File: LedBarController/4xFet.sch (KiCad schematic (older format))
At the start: 4 parts, among them Q301 Si2302DS, Q302 Si2302DS, Q303 Si2302DS, Q304 Si2302DS

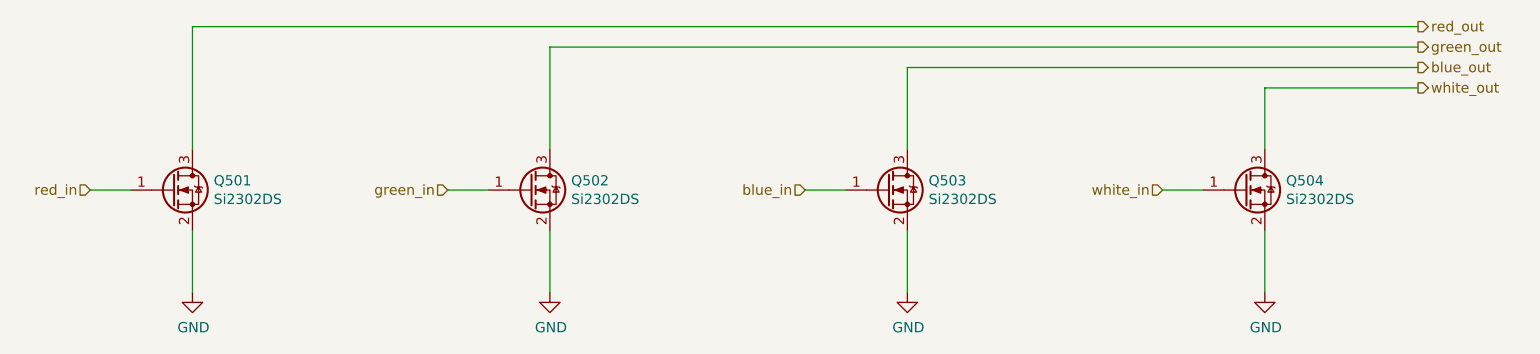
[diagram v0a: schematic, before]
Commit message: Just before reverse order of strips
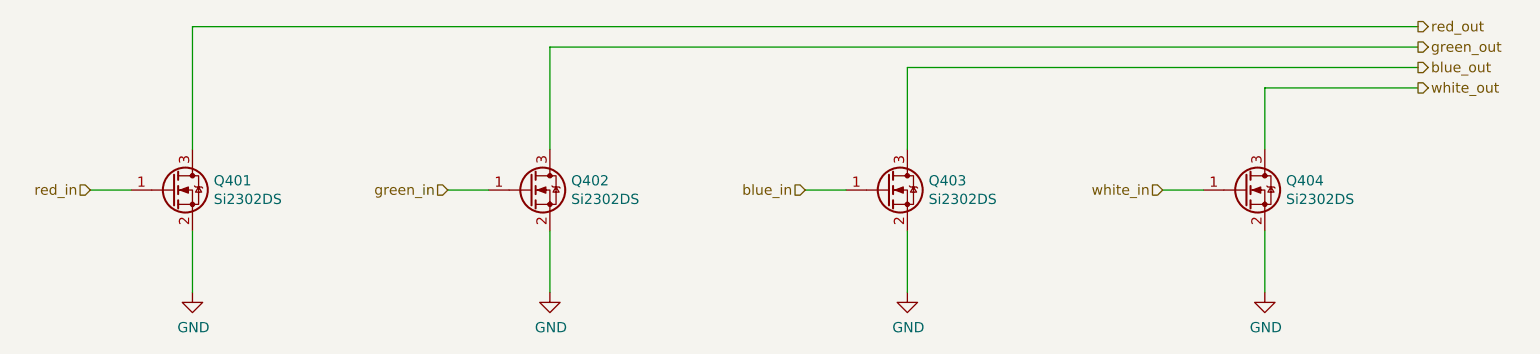
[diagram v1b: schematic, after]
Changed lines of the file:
@@
 $Descr A4 11693 8268
 encoding utf-8
-Sheet 5 13
+Sheet 4 13
 Title ""
 Date ""
@@
 AR Path="/5F8F2E1B/5F902D83/5F88FE87" Ref="#PWR0504"  Part="1"
 AR Path="/5F8F2E1B/5F902E61/5F88FE87" Ref="#PWR0604"  Part="1"
-F 0 "#PWR0604" H 7750 4050 50  0001 C CNN
+F 0 "#PWR0404" H 7750 4050 50  0001 C CNN
 F 1 "GND" H 7755 4127 50  0000 C CNN
 F 2 "" H 7750 4300 50  0001 C CNN
@@
 AR Path="/5F8F2E1B/5F902D83/5F88FE81" Ref="Q504"  Part="1"
 AR Path="/5F8F2E1B/5F902E61/5F88FE81" Ref="Q604"  Part="1"
-F 0 "Q504" H 7854 3846 50  0000 L CNN
+F 0 "Q404" H 7854 3846 50  0000 L CNN
 F 1 "Si2302DS" H 7854 3755 50  0000 L CNN
 F 2 "Package_TO_SOT_SMD:SOT-23_Handsoldering" H 7850 3900 50  0001 C CNN
@@
 AR Path="/5F8F2E1B/5F902D83/5F88FE79" Ref="#PWR0503"  Part="1"
 AR Path="/5F8F2E1B/5F902E61/5F88FE79" Ref="#PWR0603"  Part="1"
-F 0 "#PWR0603" H 6000 4050 50  0001 C CNN
+F 0 "#PWR0403" H 6000 4050 50  0001 C CNN
 F 1 "GND" H 6005 4127 50  0000 C CNN
 F 2 "" H 6000 4300 50  0001 C CNN
@@
 AR Path="/5F8F2E1B/5F902D83/5F88FE73" Ref="Q503"  Part="1"
 AR Path="/5F8F2E1B/5F902E61/5F88FE73" Ref="Q603"  Part="1"
-F 0 "Q503" H 6104 3846 50  0000 L CNN
+F 0 "Q403" H 6104 3846 50  0000 L CNN
 F 1 "Si2302DS" H 6104 3755 50  0000 L CNN
 F 2 "Package_TO_SOT_SMD:SOT-23_Handsoldering" H 6100 3900 50  0001 C CNN
@@
 AR Path="/5F8F2E1B/5F902D83/5F88FE6B" Ref="#PWR0502"  Part="1"
 AR Path="/5F8F2E1B/5F902E61/5F88FE6B" Ref="#PWR0602"  Part="1"
-F 0 "#PWR0602" H 4250 4050 50  0001 C CNN
+F 0 "#PWR0402" H 4250 4050 50  0001 C CNN
 F 1 "GND" H 4255 4127 50  0000 C CNN
 F 2 "" H 4250 4300 50  0001 C CNN
@@
 AR Path="/5F8F2E1B/5F902D83/5F88FE65" Ref="Q502"  Part="1"
 AR Path="/5F8F2E1B/5F902E61/5F88FE65" Ref="Q602"  Part="1"
-F 0 "Q502" H 4354 3846 50  0000 L CNN
+F 0 "Q402" H 4354 3846 50  0000 L CNN
 F 1 "Si2302DS" H 4354 3755 50  0000 L CNN
 F 2 "Package_TO_SOT_SMD:SOT-23_Handsoldering" H 4350 3900 50  0001 C CNN
@@
 AR Path="/5F8F2E1B/5F902D83/5F88FE5E" Ref="#PWR0501"  Part="1"
 AR Path="/5F8F2E1B/5F902E61/5F88FE5E" Ref="#PWR0601"  Part="1"
-F 0 "#PWR0601" H 2500 4050 50  0001 C CNN
+F 0 "#PWR0401" H 2500 4050 50  0001 C CNN
 F 1 "GND" H 2505 4127 50  0000 C CNN
 F 2 "" H 2500 4300 50  0001 C CNN
@@
 AR Path="/5F8F2E1B/5F902D83/5F88FE58" Ref="Q501"  Part="1"
 AR Path="/5F8F2E1B/5F902E61/5F88FE58" Ref="Q601"  Part="1"
-F 0 "Q501" H 2604 3846 50  0000 L CNN
+F 0 "Q401" H 2604 3846 50  0000 L CNN
 F 1 "Si2302DS" H 2604 3755 50  0000 L CNN
 F 2 "Package_TO_SOT_SMD:SOT-23_Handsoldering" H 2600 3900 50  0001 C CNN

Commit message: Before moving down the center connector
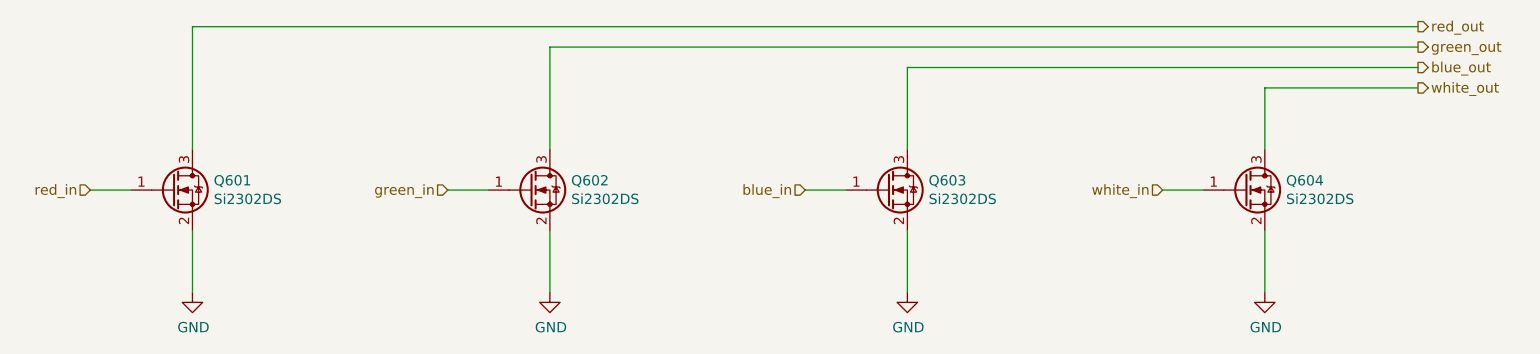
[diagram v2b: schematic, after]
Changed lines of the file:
@@
 $Descr A4 11693 8268
 encoding utf-8
-Sheet 4 13
+Sheet 6 13
 Title ""
 Date ""
@@
 AR Path="/5F8F2E1B/5F902D83/5F88FE87" Ref="#PWR0504"  Part="1"
 AR Path="/5F8F2E1B/5F902E61/5F88FE87" Ref="#PWR0604"  Part="1"
-F 0 "#PWR0404" H 7750 4050 50  0001 C CNN
+F 0 "#PWR0604" H 7750 4050 50  0001 C CNN
 F 1 "GND" H 7755 4127 50  0000 C CNN
 F 2 "" H 7750 4300 50  0001 C CNN
@@
 AR Path="/5F8F2E1B/5F902D83/5F88FE81" Ref="Q504"  Part="1"
 AR Path="/5F8F2E1B/5F902E61/5F88FE81" Ref="Q604"  Part="1"
-F 0 "Q404" H 7854 3846 50  0000 L CNN
+F 0 "Q604" H 7854 3846 50  0000 L CNN
 F 1 "Si2302DS" H 7854 3755 50  0000 L CNN
 F 2 "Package_TO_SOT_SMD:SOT-23_Handsoldering" H 7850 3900 50  0001 C CNN
@@
 AR Path="/5F8F2E1B/5F902D83/5F88FE79" Ref="#PWR0503"  Part="1"
 AR Path="/5F8F2E1B/5F902E61/5F88FE79" Ref="#PWR0603"  Part="1"
-F 0 "#PWR0403" H 6000 4050 50  0001 C CNN
+F 0 "#PWR0603" H 6000 4050 50  0001 C CNN
 F 1 "GND" H 6005 4127 50  0000 C CNN
 F 2 "" H 6000 4300 50  0001 C CNN
@@
 AR Path="/5F8F2E1B/5F902D83/5F88FE73" Ref="Q503"  Part="1"
 AR Path="/5F8F2E1B/5F902E61/5F88FE73" Ref="Q603"  Part="1"
-F 0 "Q403" H 6104 3846 50  0000 L CNN
+F 0 "Q603" H 6104 3846 50  0000 L CNN
 F 1 "Si2302DS" H 6104 3755 50  0000 L CNN
 F 2 "Package_TO_SOT_SMD:SOT-23_Handsoldering" H 6100 3900 50  0001 C CNN
@@
 AR Path="/5F8F2E1B/5F902D83/5F88FE6B" Ref="#PWR0502"  Part="1"
 AR Path="/5F8F2E1B/5F902E61/5F88FE6B" Ref="#PWR0602"  Part="1"
-F 0 "#PWR0402" H 4250 4050 50  0001 C CNN
+F 0 "#PWR0602" H 4250 4050 50  0001 C CNN
 F 1 "GND" H 4255 4127 50  0000 C CNN
 F 2 "" H 4250 4300 50  0001 C CNN
@@
 AR Path="/5F8F2E1B/5F902D83/5F88FE65" Ref="Q502"  Part="1"
 AR Path="/5F8F2E1B/5F902E61/5F88FE65" Ref="Q602"  Part="1"
-F 0 "Q402" H 4354 3846 50  0000 L CNN
+F 0 "Q602" H 4354 3846 50  0000 L CNN
 F 1 "Si2302DS" H 4354 3755 50  0000 L CNN
 F 2 "Package_TO_SOT_SMD:SOT-23_Handsoldering" H 4350 3900 50  0001 C CNN
@@
 AR Path="/5F8F2E1B/5F902D83/5F88FE5E" Ref="#PWR0501"  Part="1"
 AR Path="/5F8F2E1B/5F902E61/5F88FE5E" Ref="#PWR0601"  Part="1"
-F 0 "#PWR0401" H 2500 4050 50  0001 C CNN
+F 0 "#PWR0601" H 2500 4050 50  0001 C CNN
 F 1 "GND" H 2505 4127 50  0000 C CNN
 F 2 "" H 2500 4300 50  0001 C CNN
@@
 AR Path="/5F8F2E1B/5F902D83/5F88FE58" Ref="Q501"  Part="1"
 AR Path="/5F8F2E1B/5F902E61/5F88FE58" Ref="Q601"  Part="1"
-F 0 "Q401" H 2604 3846 50  0000 L CNN
+F 0 "Q601" H 2604 3846 50  0000 L CNN
 F 1 "Si2302DS" H 2604 3755 50  0000 L CNN
 F 2 "Package_TO_SOT_SMD:SOT-23_Handsoldering" H 2600 3900 50  0001 C CNN

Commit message: Pwm circuit routed (no plane yet)
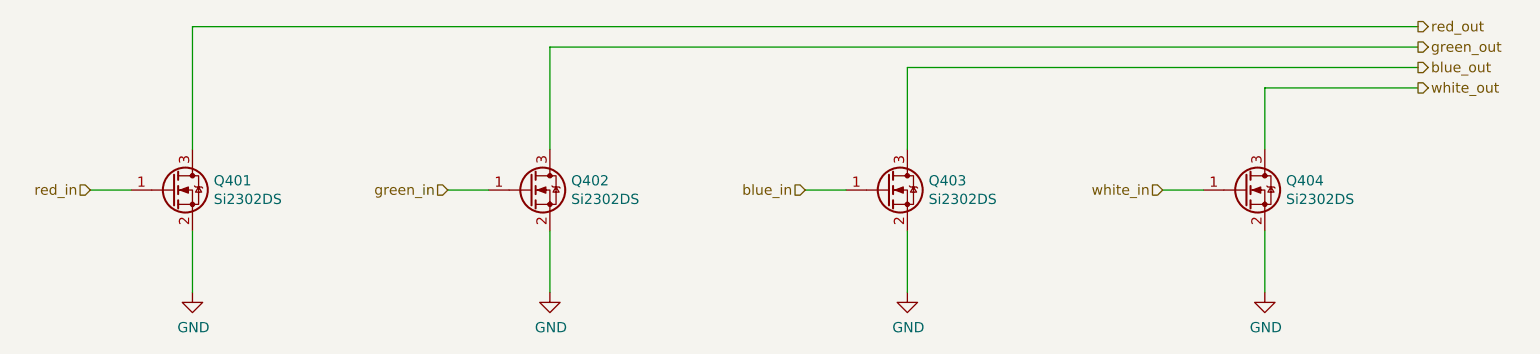
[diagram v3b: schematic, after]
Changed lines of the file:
@@
 $Descr A4 11693 8268
 encoding utf-8
-Sheet 6 13
+Sheet 4 13
 Title ""
 Date ""
@@
 AR Path="/5F8F2E1B/5F902D83/5F88FE81" Ref="Q504"  Part="1"
 AR Path="/5F8F2E1B/5F902E61/5F88FE81" Ref="Q604"  Part="1"
-F 0 "Q604" H 7854 3846 50  0000 L CNN
+F 0 "Q404" H 7854 3846 50  0000 L CNN
 F 1 "Si2302DS" H 7854 3755 50  0000 L CNN
 F 2 "Package_TO_SOT_SMD:SOT-23_Handsoldering" H 7850 3900 50  0001 C CNN
@@
 AR Path="/5F8F2E1B/5F902D83/5F88FE73" Ref="Q503"  Part="1"
 AR Path="/5F8F2E1B/5F902E61/5F88FE73" Ref="Q603"  Part="1"
-F 0 "Q603" H 6104 3846 50  0000 L CNN
+F 0 "Q403" H 6104 3846 50  0000 L CNN
 F 1 "Si2302DS" H 6104 3755 50  0000 L CNN
 F 2 "Package_TO_SOT_SMD:SOT-23_Handsoldering" H 6100 3900 50  0001 C CNN
@@
 AR Path="/5F8F2E1B/5F902D83/5F88FE65" Ref="Q502"  Part="1"
 AR Path="/5F8F2E1B/5F902E61/5F88FE65" Ref="Q602"  Part="1"
-F 0 "Q602" H 4354 3846 50  0000 L CNN
+F 0 "Q402" H 4354 3846 50  0000 L CNN
 F 1 "Si2302DS" H 4354 3755 50  0000 L CNN
 F 2 "Package_TO_SOT_SMD:SOT-23_Handsoldering" H 4350 3900 50  0001 C CNN
@@
 AR Path="/5F8F2E1B/5F902D83/5F88FE58" Ref="Q501"  Part="1"
 AR Path="/5F8F2E1B/5F902E61/5F88FE58" Ref="Q601"  Part="1"
-F 0 "Q601" H 2604 3846 50  0000 L CNN
+F 0 "Q401" H 2604 3846 50  0000 L CNN
 F 1 "Si2302DS" H 2604 3755 50  0000 L CNN
 F 2 "Package_TO_SOT_SMD:SOT-23_Handsoldering" H 2600 3900 50  0001 C CNN

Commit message: Added fill zones
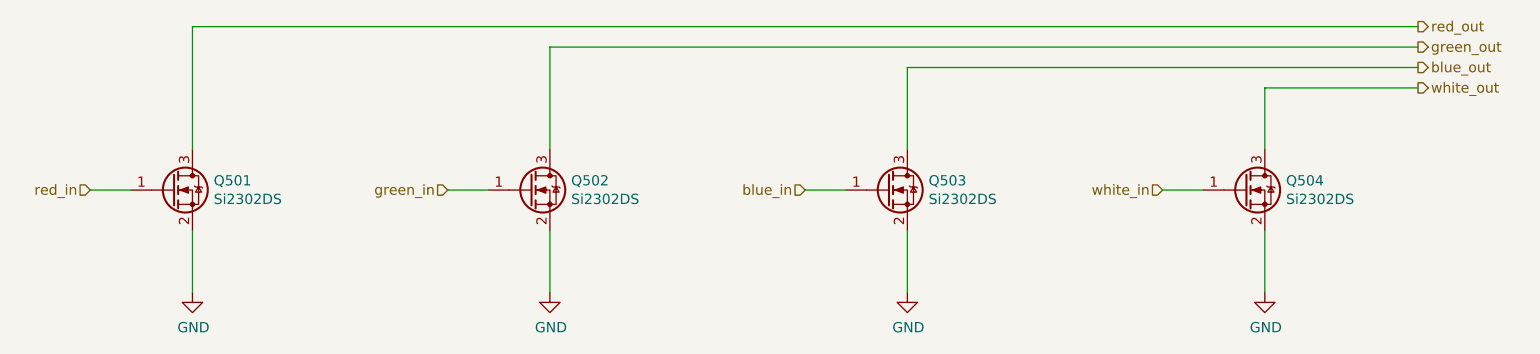
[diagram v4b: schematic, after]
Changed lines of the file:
@@
 $Descr A4 11693 8268
 encoding utf-8
-Sheet 4 13
+Sheet 5 13
 Title ""
 Date ""
@@
 AR Path="/5F8F2E1B/5F902D83/5F88FE87" Ref="#PWR0504"  Part="1"
 AR Path="/5F8F2E1B/5F902E61/5F88FE87" Ref="#PWR0604"  Part="1"
-F 0 "#PWR0604" H 7750 4050 50  0001 C CNN
+F 0 "#PWR0504" H 7750 4050 50  0001 C CNN
 F 1 "GND" H 7755 4127 50  0000 C CNN
 F 2 "" H 7750 4300 50  0001 C CNN
@@
 AR Path="/5F8F2E1B/5F902D83/5F88FE81" Ref="Q504"  Part="1"
 AR Path="/5F8F2E1B/5F902E61/5F88FE81" Ref="Q604"  Part="1"
-F 0 "Q404" H 7854 3846 50  0000 L CNN
+F 0 "Q504" H 7854 3846 50  0000 L CNN
 F 1 "Si2302DS" H 7854 3755 50  0000 L CNN
 F 2 "Package_TO_SOT_SMD:SOT-23_Handsoldering" H 7850 3900 50  0001 C CNN
@@
 AR Path="/5F8F2E1B/5F902D83/5F88FE79" Ref="#PWR0503"  Part="1"
 AR Path="/5F8F2E1B/5F902E61/5F88FE79" Ref="#PWR0603"  Part="1"
-F 0 "#PWR0603" H 6000 4050 50  0001 C CNN
+F 0 "#PWR0503" H 6000 4050 50  0001 C CNN
 F 1 "GND" H 6005 4127 50  0000 C CNN
 F 2 "" H 6000 4300 50  0001 C CNN
@@
 AR Path="/5F8F2E1B/5F902D83/5F88FE73" Ref="Q503"  Part="1"
 AR Path="/5F8F2E1B/5F902E61/5F88FE73" Ref="Q603"  Part="1"
-F 0 "Q403" H 6104 3846 50  0000 L CNN
+F 0 "Q503" H 6104 3846 50  0000 L CNN
 F 1 "Si2302DS" H 6104 3755 50  0000 L CNN
 F 2 "Package_TO_SOT_SMD:SOT-23_Handsoldering" H 6100 3900 50  0001 C CNN
@@
 AR Path="/5F8F2E1B/5F902D83/5F88FE6B" Ref="#PWR0502"  Part="1"
 AR Path="/5F8F2E1B/5F902E61/5F88FE6B" Ref="#PWR0602"  Part="1"
-F 0 "#PWR0602" H 4250 4050 50  0001 C CNN
+F 0 "#PWR0502" H 4250 4050 50  0001 C CNN
 F 1 "GND" H 4255 4127 50  0000 C CNN
 F 2 "" H 4250 4300 50  0001 C CNN
@@
 AR Path="/5F8F2E1B/5F902D83/5F88FE65" Ref="Q502"  Part="1"
 AR Path="/5F8F2E1B/5F902E61/5F88FE65" Ref="Q602"  Part="1"
-F 0 "Q402" H 4354 3846 50  0000 L CNN
+F 0 "Q502" H 4354 3846 50  0000 L CNN
 F 1 "Si2302DS" H 4354 3755 50  0000 L CNN
 F 2 "Package_TO_SOT_SMD:SOT-23_Handsoldering" H 4350 3900 50  0001 C CNN
@@
 AR Path="/5F8F2E1B/5F902D83/5F88FE5E" Ref="#PWR0501"  Part="1"
 AR Path="/5F8F2E1B/5F902E61/5F88FE5E" Ref="#PWR0601"  Part="1"
-F 0 "#PWR0601" H 2500 4050 50  0001 C CNN
+F 0 "#PWR0501" H 2500 4050 50  0001 C CNN
 F 1 "GND" H 2505 4127 50  0000 C CNN
 F 2 "" H 2500 4300 50  0001 C CNN
@@
 AR Path="/5F8F2E1B/5F902D83/5F88FE58" Ref="Q501"  Part="1"
 AR Path="/5F8F2E1B/5F902E61/5F88FE58" Ref="Q601"  Part="1"
-F 0 "Q401" H 2604 3846 50  0000 L CNN
+F 0 "Q501" H 2604 3846 50  0000 L CNN
 F 1 "Si2302DS" H 2604 3755 50  0000 L CNN
 F 2 "Package_TO_SOT_SMD:SOT-23_Handsoldering" H 2600 3900 50  0001 C CNN
